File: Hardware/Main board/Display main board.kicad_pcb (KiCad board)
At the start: 2 copper layers, 142.2 x 91.4 mm, 86 parts, among them J1 Board to Board, J2 BATT JST, J3 Conn_ARM_SWD_TagConnect_TC203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, P1 USB_C_Plug_USB2.0, SW1 USB BOOT, U1 BQ25895, U10 ABM8-272-T3, U2 W25Q32JVSS, U3 TS3USB221A, U4 AP7361C-33E, U5 AP7361C-33E, U6 AP7361C-33E, U7 AP7361C-33E, U8 TPM8837C, U9 RP2040

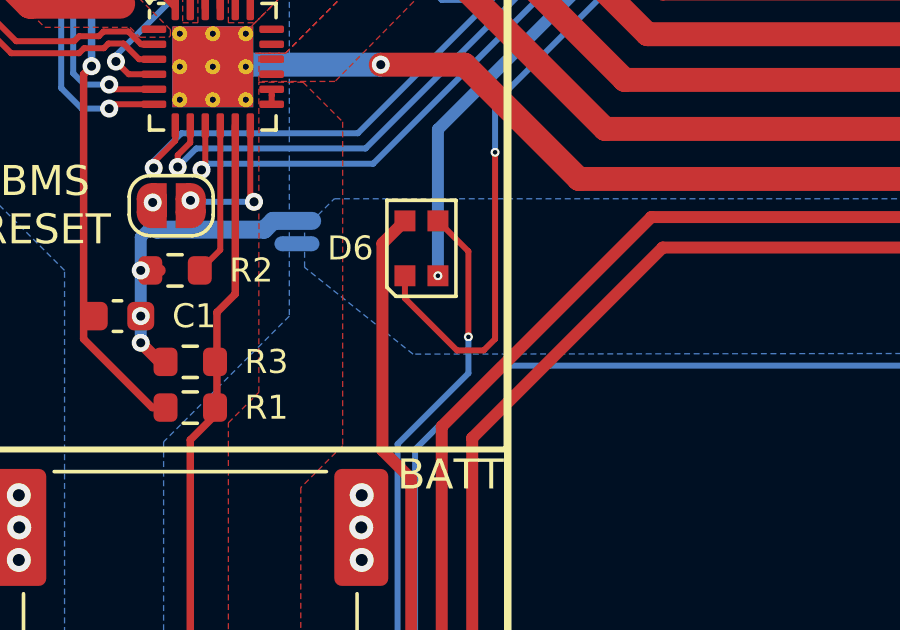
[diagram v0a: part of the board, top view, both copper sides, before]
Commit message: update constraints
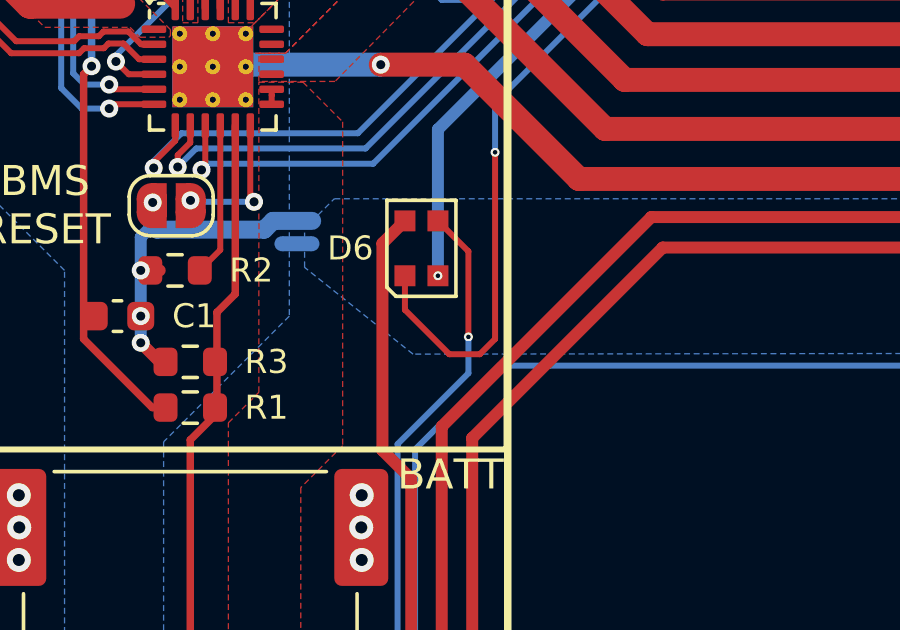
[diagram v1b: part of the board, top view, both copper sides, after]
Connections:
- D2 pad 3: Net-(D2-DIN) -> unconnected-(D2-DIN-Pad3)
- U9 pad 13: Net-(D2-DIN) -> unconnected-(U9-GPIO10-Pad13)
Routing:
- net Net-(D2-DIN): track 13.5 -> 0.00 mm, vias 2 -> 0
- net (no net): track 0.00 -> 13.5 mm, vias 6 -> 8
